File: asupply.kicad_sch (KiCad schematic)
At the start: 93 parts

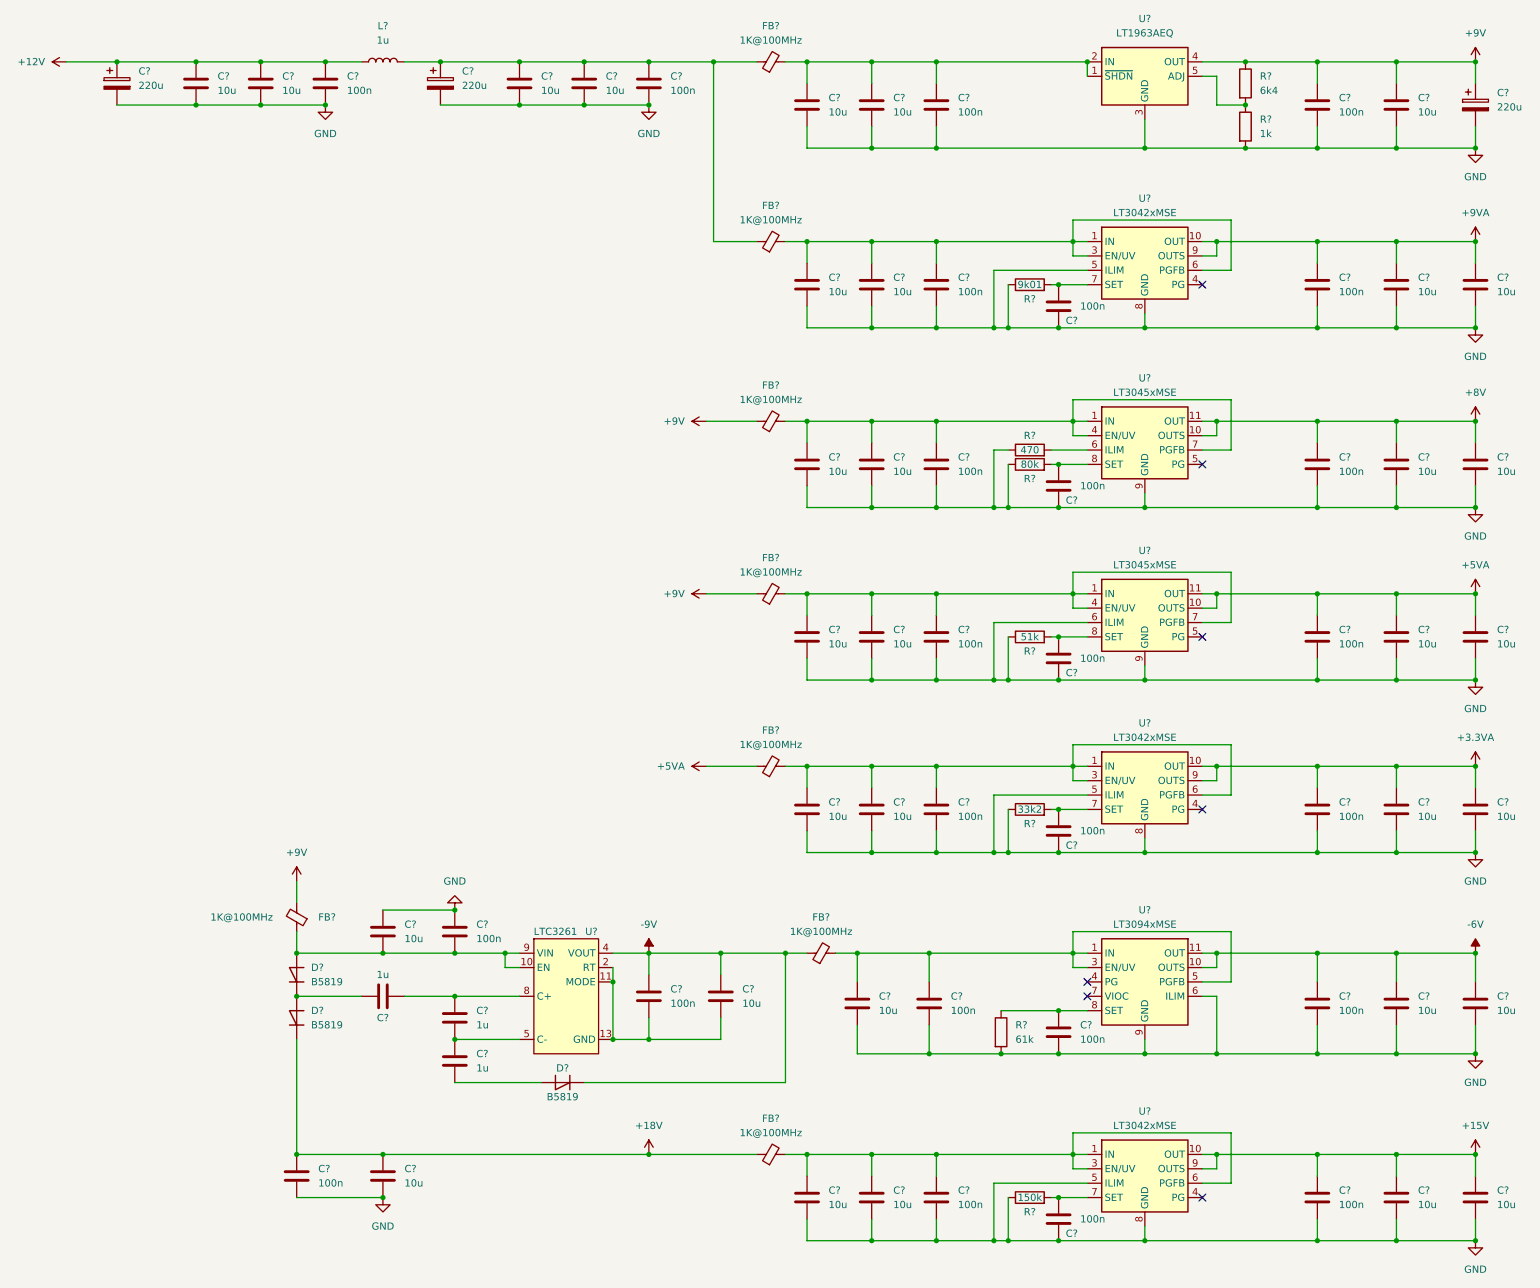
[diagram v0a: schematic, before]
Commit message: complete mcu
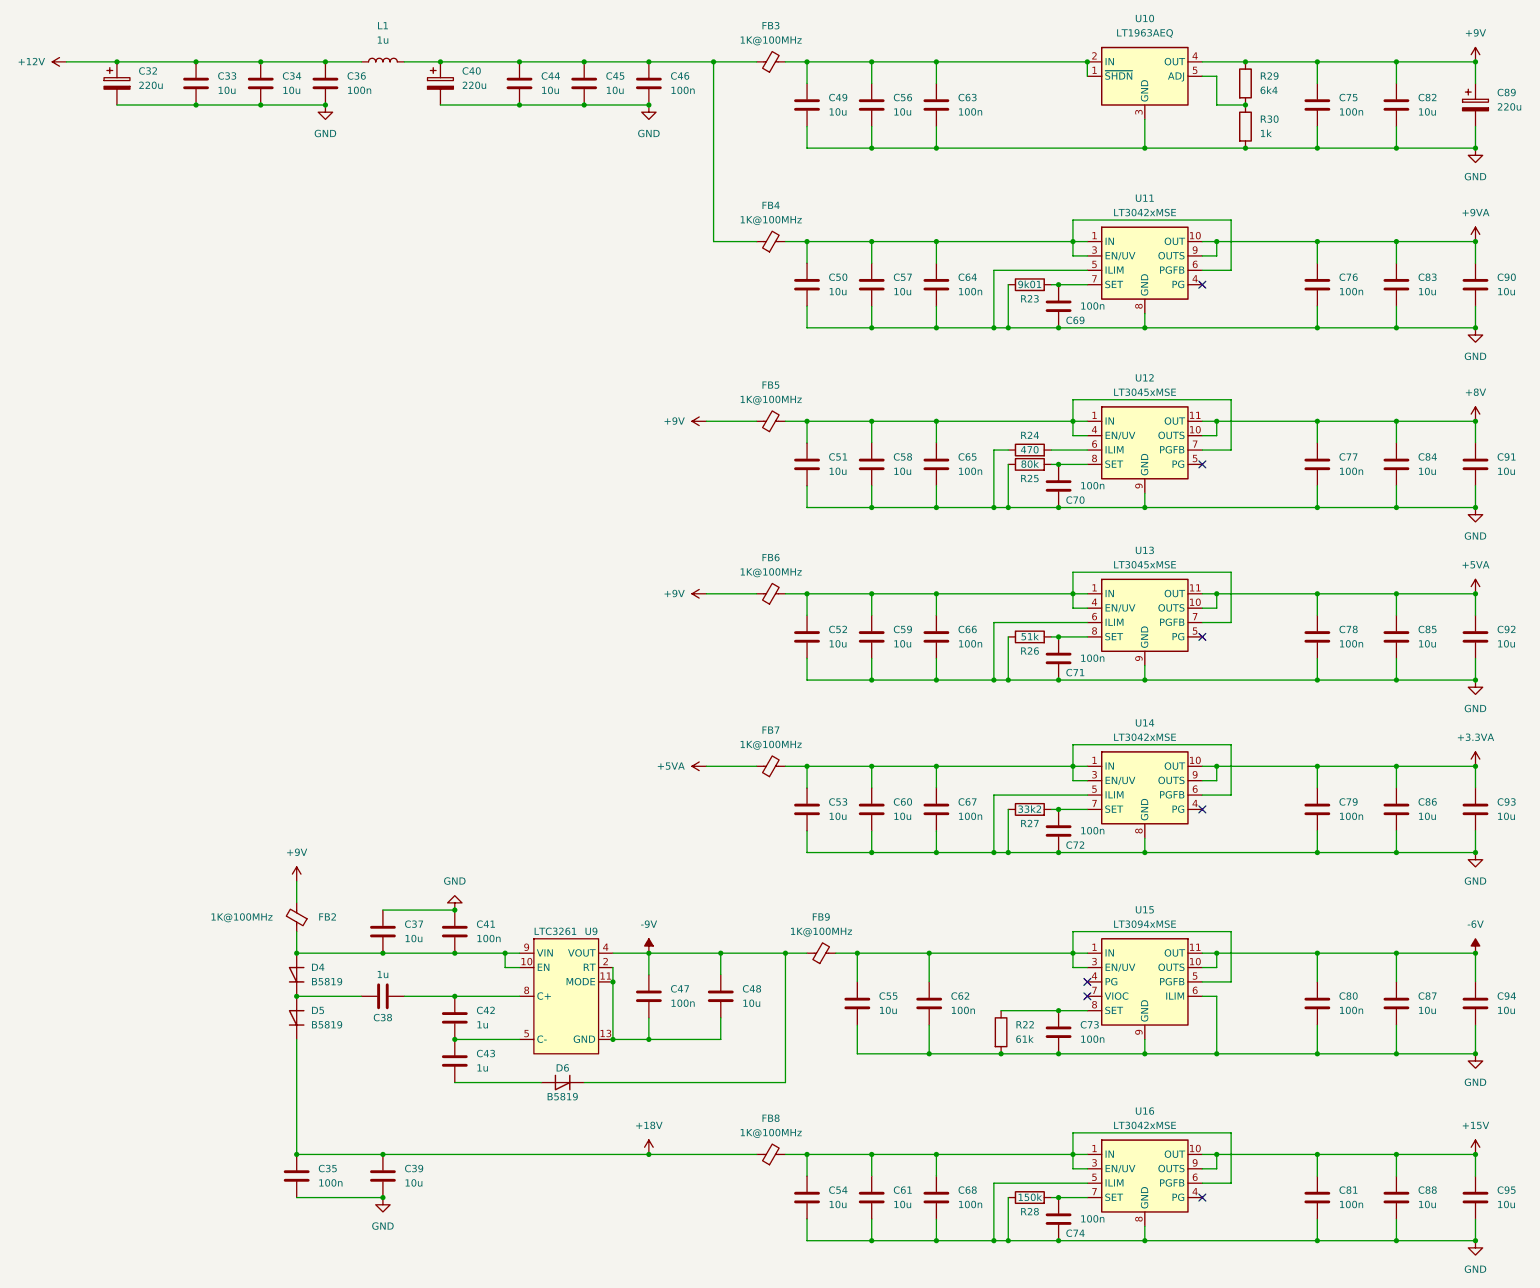
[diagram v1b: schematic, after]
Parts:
- gave numbers to parts that had none: 93
